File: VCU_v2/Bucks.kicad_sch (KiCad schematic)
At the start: 16 parts, among them U2 TPS5430

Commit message: bspd schematic done
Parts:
- D4: LCSC P/N (none) -> C125093
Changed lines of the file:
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@@
+			)
+		)
+		(property "LCSC P/N" "C125093"
+			(at 222.25 59.69 90)
+			(effects
+				(font
+					(size 1.27 1.27)
+				)
+				(hide yes)
 			)
 		)

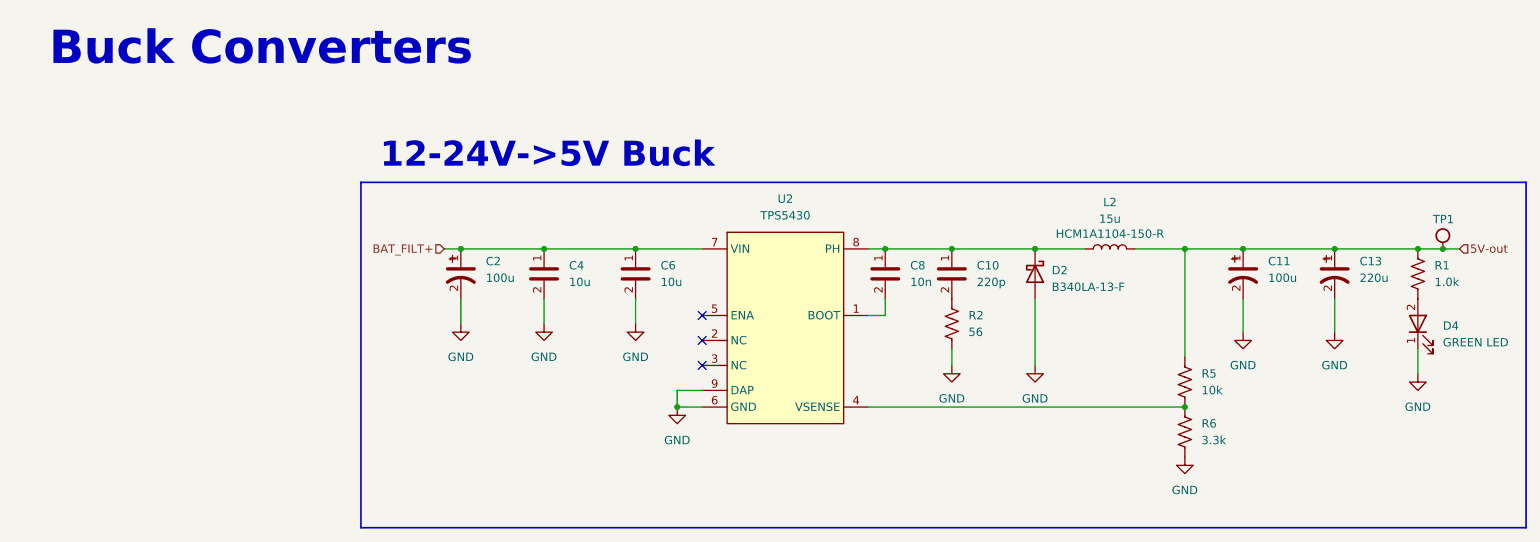
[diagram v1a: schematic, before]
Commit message: vcu v2 schematics done
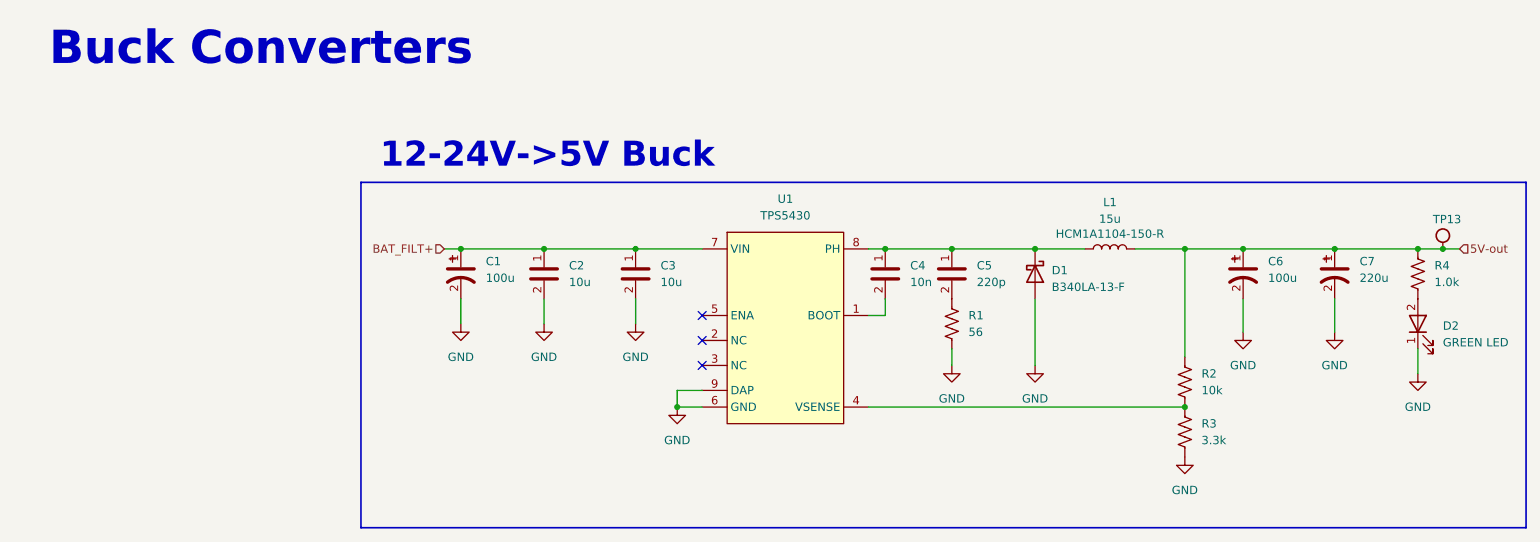
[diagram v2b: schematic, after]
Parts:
- renumbered C2 to C1, C4 to C2, C6 to C3, C8 to C4, C10 to C5, C11 to C6, C13 to C7, D2 to D1, D4 to D2, L2 to L1, R2 to R1, R5 to R2, R6 to R3, R1 to R4, TP1 to TP13, U2 to U1
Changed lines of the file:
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@@
 		(dnp no)
 		(fields_autoplaced yes)
-		(property "Reference" "#PWR023"
+		(property "Reference" "#PWR017"
 			(at 186.69 86.36 0)
 			(effects
@@
 			(project ""
 				(path "/4ee6c2ad-9a1b-4276-b3cf-1cc8dc52967e/9e4b5f8d-93dc-46d5-aa92-d0e0d2e07b3d/83ba1e49-760f-4968-9bbd-ff2e6c9ab433"
-					(reference "#PWR023")
+					(reference "#PWR017")
 					(unit 1)
 				)
@@
 		(dnp no)
 		(fields_autoplaced yes)
-		(property "Reference" "#PWR021"
+		(property "Reference" "#PWR016"
 			(at 163.83 72.39 0)
 			(effects
@@
 			(project "VCU_v1"
 				(path "/4ee6c2ad-9a1b-4276-b3cf-1cc8dc52967e/9e4b5f8d-93dc-46d5-aa92-d0e0d2e07b3d/83ba1e49-760f-4968-9bbd-ff2e6c9ab433"
-					(reference "#PWR021")
+					(reference "#PWR016")
 					(unit 1)
 				)
@@
 		(dnp no)
 		(fields_autoplaced yes)
-		(property "Reference" "#PWR013"
+		(property "Reference" "#PWR012"
 			(at 88.9 66.04 0)
 			(effects
@@
 			(project "VCU_v1"
 				(path "/4ee6c2ad-9a1b-4276-b3cf-1cc8dc52967e/9e4b5f8d-93dc-46d5-aa92-d0e0d2e07b3d/83ba1e49-760f-4968-9bbd-ff2e6c9ab433"
-					(reference "#PWR013")
+					(reference "#PWR012")
 					(unit 1)
 				)
@@
 		(dnp no)
 		(fields_autoplaced yes)
-		(property "Reference" "C6"
+		(property "Reference" "C3"
 			(at 106.68 50.7999 0)
 			(effects
@@
 			(project "VCU_v1"
 				(path "/4ee6c2ad-9a1b-4276-b3cf-1cc8dc52967e/9e4b5f8d-93dc-46d5-aa92-d0e0d2e07b3d/83ba1e49-760f-4968-9bbd-ff2e6c9ab433"
-					(reference "C6")
+					(reference "C3")
 					(unit 1)
 				)
@@
 		(on_board yes)
 		(dnp no)
-		(property "Reference" "D2"
+		(property "Reference" "D1"
 			(at 166.37 50.8 90)
 			(effects
@@
 			(project "VCU_v1"
 				(path "/4ee6c2ad-9a1b-4276-b3cf-1cc8dc52967e/9e4b5f8d-93dc-46d5-aa92-d0e0d2e07b3d/83ba1e49-760f-4968-9bbd-ff2e6c9ab433"
-					(reference "D2")
+					(reference "D1")
 					(unit 1)
 				)
@@
 		(dnp no)
 		(fields_autoplaced yes)
-		(property "Reference" "R2"
+		(property "Reference" "R1"
 			(at 153.67 58.4199 90)
 			(effects
@@
 			(project ""
 				(path "/4ee6c2ad-9a1b-4276-b3cf-1cc8dc52967e/9e4b5f8d-93dc-46d5-aa92-d0e0d2e07b3d/83ba1e49-760f-4968-9bbd-ff2e6c9ab433"
-					(reference "R2")
+					(reference "R1")
 					(unit 1)
 				)
@@
 		(dnp no)
 		(fields_autoplaced yes)
-		(property "Reference" "U2"
+		(property "Reference" "U1"
 			(at 125.73 40.64 0)
 			(effects
@@
 			(project "VCU_v1"
 				(path "/4ee6c2ad-9a1b-4276-b3cf-1cc8dc52967e/9e4b5f8d-93dc-46d5-aa92-d0e0d2e07b3d/83ba1e49-760f-4968-9bbd-ff2e6c9ab433"
-					(reference "U2")
+					(reference "U1")
 					(unit 1)
 				)
@@
 		(dnp no)
 		(fields_autoplaced yes)
-		(property "Reference" "C8"
+		(property "Reference" "C4"
 			(at 144.78 50.7999 0)
 			(effects
@@
 			(project "VCU_v1"
 				(path "/4ee6c2ad-9a1b-4276-b3cf-1cc8dc52967e/9e4b5f8d-93dc-46d5-aa92-d0e0d2e07b3d/83ba1e49-760f-4968-9bbd-ff2e6c9ab433"
-					(reference "C8")
+					(reference "C4")
 					(unit 1)
 				)
@@
 		(dnp no)
 		(fields_autoplaced yes)
-		(property "Reference" "#PWR017"
+		(property "Reference" "#PWR014"
 			(at 109.22 78.74 0)
 			(effects
@@
 			(project "VCU_v1"
 				(path "/4ee6c2ad-9a1b-4276-b3cf-1cc8dc52967e/9e4b5f8d-93dc-46d5-aa92-d0e0d2e07b3d/83ba1e49-760f-4968-9bbd-ff2e6c9ab433"
-					(reference "#PWR017")
+					(reference "#PWR014")
 					(unit 1)
 				)
@@
 		(dnp no)
 		(fields_autoplaced yes)
-		(property "Reference" "#PWR019"
+		(property "Reference" "#PWR015"
 			(at 151.13 72.39 0)
 			(effects
@@
 			(project "VCU_v1"
 				(path "/4ee6c2ad-9a1b-4276-b3cf-1cc8dc52967e/9e4b5f8d-93dc-46d5-aa92-d0e0d2e07b3d/83ba1e49-760f-4968-9bbd-ff2e6c9ab433"
-					(reference "#PWR019")
+					(reference "#PWR015")
 					(unit 1)
 				)
@@
 		(on_board yes)
 		(dnp no)
-		(property "Reference" "L2"
+		(property "Reference" "L1"
 			(at 175.26 41.148 90)
 			(effects
@@
 			(project ""
 				(path "/4ee6c2ad-9a1b-4276-b3cf-1cc8dc52967e/9e4b5f8d-93dc-46d5-aa92-d0e0d2e07b3d/83ba1e49-760f-4968-9bbd-ff2e6c9ab433"
-					(reference "L2")
+					(reference "L1")
 					(unit 1)
 				)
@@
 		(dnp no)
 		(fields_autoplaced yes)
-		(property "Reference" "R6"
+		(property "Reference" "R3"
 			(at 189.23 74.9299 90)
 			(effects
@@
 			(project ""
 				(path "/4ee6c2ad-9a1b-4276-b3cf-1cc8dc52967e/9e4b5f8d-93dc-46d5-aa92-d0e0d2e07b3d/83ba1e49-760f-4968-9bbd-ff2e6c9ab433"
-					(reference "R6")
+					(reference "R3")
 					(unit 1)
 				)
@@
 		(dnp no)
 		(fields_autoplaced yes)
-		(property "Reference" "C2"
+		(property "Reference" "C1"
 			(at 80.01 50.1649 0)
 			(effects
@@
 			(project ""
 				(path "/4ee6c2ad-9a1b-4276-b3cf-1cc8dc52967e/9e4b5f8d-93dc-46d5-aa92-d0e0d2e07b3d/83ba1e49-760f-4968-9bbd-ff2e6c9ab433"
-					(reference "C2")
+					(reference "C1")
 					(unit 1)
 				)
@@
 		(dnp no)
 		(fields_autoplaced yes)
-		(property "Reference" "R5"
+		(property "Reference" "R2"
 			(at 189.23 67.3099 90)
 			(effects
@@
 			(project ""
 				(path "/4ee6c2ad-9a1b-4276-b3cf-1cc8dc52967e/9e4b5f8d-93dc-46d5-aa92-d0e0d2e07b3d/83ba1e49-760f-4968-9bbd-ff2e6c9ab433"
-					(reference "R5")
+					(reference "R2")
 					(unit 1)
 				)
@@
 		(dnp no)
 		(fields_autoplaced yes)
-		(property "Reference" "C10"
+		(property "Reference" "C5"
 			(at 154.94 50.7999 0)
 			(effects
@@
 			(project ""
 				(path "/4ee6c2ad-9a1b-4276-b3cf-1cc8dc52967e/9e4b5f8d-93dc-46d5-aa92-d0e0d2e07b3d/83ba1e49-760f-4968-9bbd-ff2e6c9ab433"
-					(reference "C10")
+					(reference "C5")
 					(unit 1)
 				)
@@
 		(dnp no)
 		(fields_autoplaced yes)
-		(property "Reference" "#PWR026"
+		(property "Reference" "#PWR019"
 			(at 209.55 67.31 0)
 			(effects
@@
 			(project "VCU_v1"
 				(path "/4ee6c2ad-9a1b-4276-b3cf-1cc8dc52967e/9e4b5f8d-93dc-46d5-aa92-d0e0d2e07b3d/83ba1e49-760f-4968-9bbd-ff2e6c9ab433"
-					(reference "#PWR026")
+					(reference "#PWR019")
 					(unit 1)
 				)
@@
 		(dnp no)
 		(fields_autoplaced yes)
-		(property "Reference" "D4"
+		(property "Reference" "D2"
 			(at 226.06 60.0074 90)
 			(effects
@@
 			(project "VCU_v1"
 				(path "/4ee6c2ad-9a1b-4276-b3cf-1cc8dc52967e/9e4b5f8d-93dc-46d5-aa92-d0e0d2e07b3d/83ba1e49-760f-4968-9bbd-ff2e6c9ab433"
-					(reference "D4")
+					(reference "D2")
 					(unit 1)
 				)
@@
 		(on_board yes)
 		(dnp no)
-		(property "Reference" "TP1"
+		(property "Reference" "TP13"
 			(at 224.5368 43.0037 0)
 			(effects
@@
 			(project "VCU_v1"
 				(path "/4ee6c2ad-9a1b-4276-b3cf-1cc8dc52967e/9e4b5f8d-93dc-46d5-aa92-d0e0d2e07b3d/83ba1e49-760f-4968-9bbd-ff2e6c9ab433"
-					(reference "TP1")
+					(reference "TP13")
 					(unit 1)
 				)
@@
 		(dnp no)
 		(fields_autoplaced yes)
-		(property "Reference" "#PWR024"
+		(property "Reference" "#PWR018"
 			(at 195.58 67.31 0)
 			(effects
@@
 			(project "VCU_v1"
 				(path "/4ee6c2ad-9a1b-4276-b3cf-1cc8dc52967e/9e4b5f8d-93dc-46d5-aa92-d0e0d2e07b3d/83ba1e49-760f-4968-9bbd-ff2e6c9ab433"
-					(reference "#PWR024")
+					(reference "#PWR018")
 					(unit 1)
 				)
@@
 		(dnp no)
 		(fields_autoplaced yes)
-		(property "Reference" "C4"
+		(property "Reference" "C2"
 			(at 92.71 50.7999 0)
 			(effects
@@
 			(project "VCU_v1"
 				(path "/4ee6c2ad-9a1b-4276-b3cf-1cc8dc52967e/9e4b5f8d-93dc-46d5-aa92-d0e0d2e07b3d/83ba1e49-760f-4968-9bbd-ff2e6c9ab433"
-					(reference "C4")
+					(reference "C2")
 					(unit 1)
 				)
@@
 		(dnp no)
 		(fields_autoplaced yes)
-		(property "Reference" "#PWR028"
+		(property "Reference" "#PWR020"
 			(at 222.25 73.66 0)
 			(effects
@@
 			(project "VCU_v1"
 				(path "/4ee6c2ad-9a1b-4276-b3cf-1cc8dc52967e/9e4b5f8d-93dc-46d5-aa92-d0e0d2e07b3d/83ba1e49-760f-4968-9bbd-ff2e6c9ab433"
-					(reference "#PWR028")
+					(reference "#PWR020")
 					(unit 1)
 				)
@@
 		(dnp no)
 		(fields_autoplaced yes)
-		(property "Reference" "C13"
+		(property "Reference" "C7"
 			(at 213.36 50.1649 0)
 			(effects
@@
 			(project ""
 				(path "/4ee6c2ad-9a1b-4276-b3cf-1cc8dc52967e/9e4b5f8d-93dc-46d5-aa92-d0e0d2e07b3d/83ba1e49-760f-4968-9bbd-ff2e6c9ab433"
-					(reference "C13")
+					(reference "C7")
 					(unit 1)
 				)
@@
 		(dnp no)
 		(fields_autoplaced yes)
-		(property "Reference" "R1"
+		(property "Reference" "R4"
 			(at 224.79 50.7999 90)
 			(effects
@@
 			(project ""
 				(path "/4ee6c2ad-9a1b-4276-b3cf-1cc8dc52967e/9e4b5f8d-93dc-46d5-aa92-d0e0d2e07b3d/83ba1e49-760f-4968-9bbd-ff2e6c9ab433"
-					(reference "R1")
+					(reference "R4")
 					(unit 1)
 				)
@@
 		(dnp no)
 		(fields_autoplaced yes)
-		(property "Reference" "C11"
+		(property "Reference" "C6"
 			(at 199.39 50.1649 0)
 			(effects
@@
 			(project ""
 				(path "/4ee6c2ad-9a1b-4276-b3cf-1cc8dc52967e/9e4b5f8d-93dc-46d5-aa92-d0e0d2e07b3d/83ba1e49-760f-4968-9bbd-ff2e6c9ab433"
-					(reference "C11")
+					(reference "C6")
 					(unit 1)
 				)
@@
 		(dnp no)
 		(fields_autoplaced yes)
-		(property "Reference" "#PWR015"
+		(property "Reference" "#PWR013"
 			(at 102.87 66.04 0)
 			(effects
@@
 			(project "VCU_v1"
 				(path "/4ee6c2ad-9a1b-4276-b3cf-1cc8dc52967e/9e4b5f8d-93dc-46d5-aa92-d0e0d2e07b3d/83ba1e49-760f-4968-9bbd-ff2e6c9ab433"
-					(reference "#PWR015")
+					(reference "#PWR013")
 					(unit 1)
 				)
